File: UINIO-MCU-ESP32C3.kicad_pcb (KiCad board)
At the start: 2 copper layers, 59.8 x 20.4 mm, 50 parts, among them J1 Conn_01x15_Male, J2 外接串行下载接口, J3 Conn_01x15_Male, SW1 复位按键, SW2 下载按键, U1 ME6211C33M5G-N, U2 W25Q128JVSSIQ, U3 ESP32-C3, U4 CH343P, Y1 40MHz

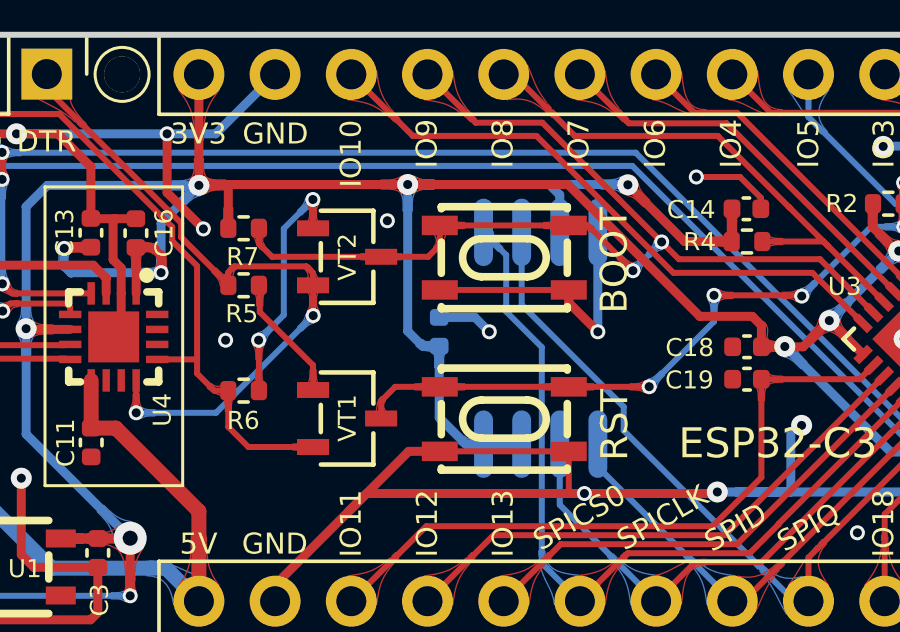
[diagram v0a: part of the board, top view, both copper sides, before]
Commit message: Release UINIO-MCU-ESP32C3 version 3.0.0.
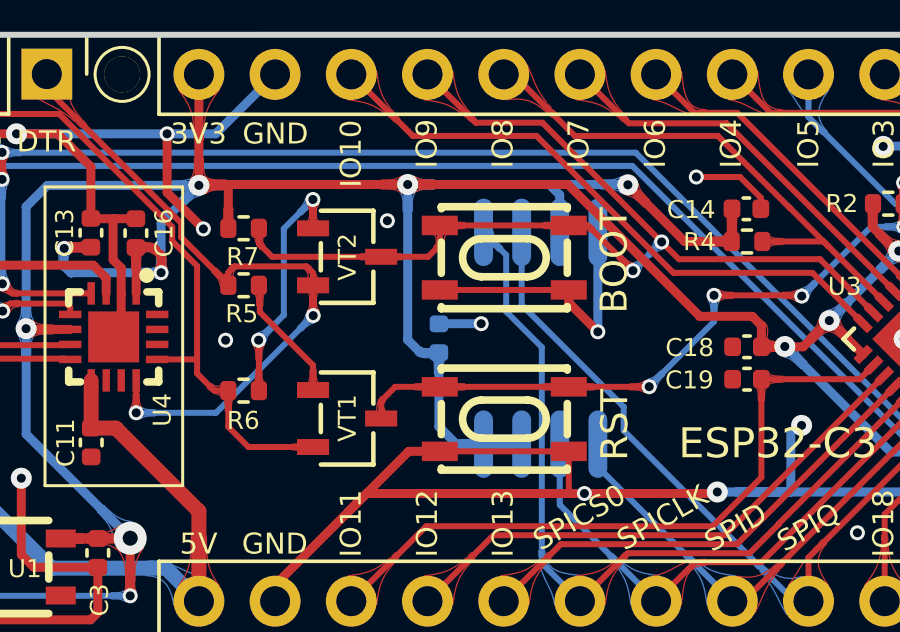
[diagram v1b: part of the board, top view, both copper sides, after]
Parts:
- moved C1 0.22 mm to (146.2, 103.0)

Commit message: Release UINIO-MCU-ESP32C3 version 3.0.0.
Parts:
- moved ? 0.06 mm to (141.7, 103.1)
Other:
- board text added: "ADC1 IO4/SDA"
- board text added: "ADC2 IO5/SCL"
- board text removed: "ADC1 IO4 SDA"
- board text removed: "ADC2 IO5 SCL"
